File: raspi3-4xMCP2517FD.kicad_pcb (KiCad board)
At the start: 2 copper layers, 25.4 x 53.3 mm, 44 parts, among them J1 Raspberry_Pi_2_3, J2 Conn_02x04_Odd_Even, U1 MCP2517FD-xSL, U2 MCP2517FD-xSL, U3 MCP2517FD-xSL, U4 MCP2517FD-xSL, U5 TJA1049T-3, U6 TJA1049T-3, U7 TJA1049T-3, U8 TJA1049T-3, X1 ASV-20MHz

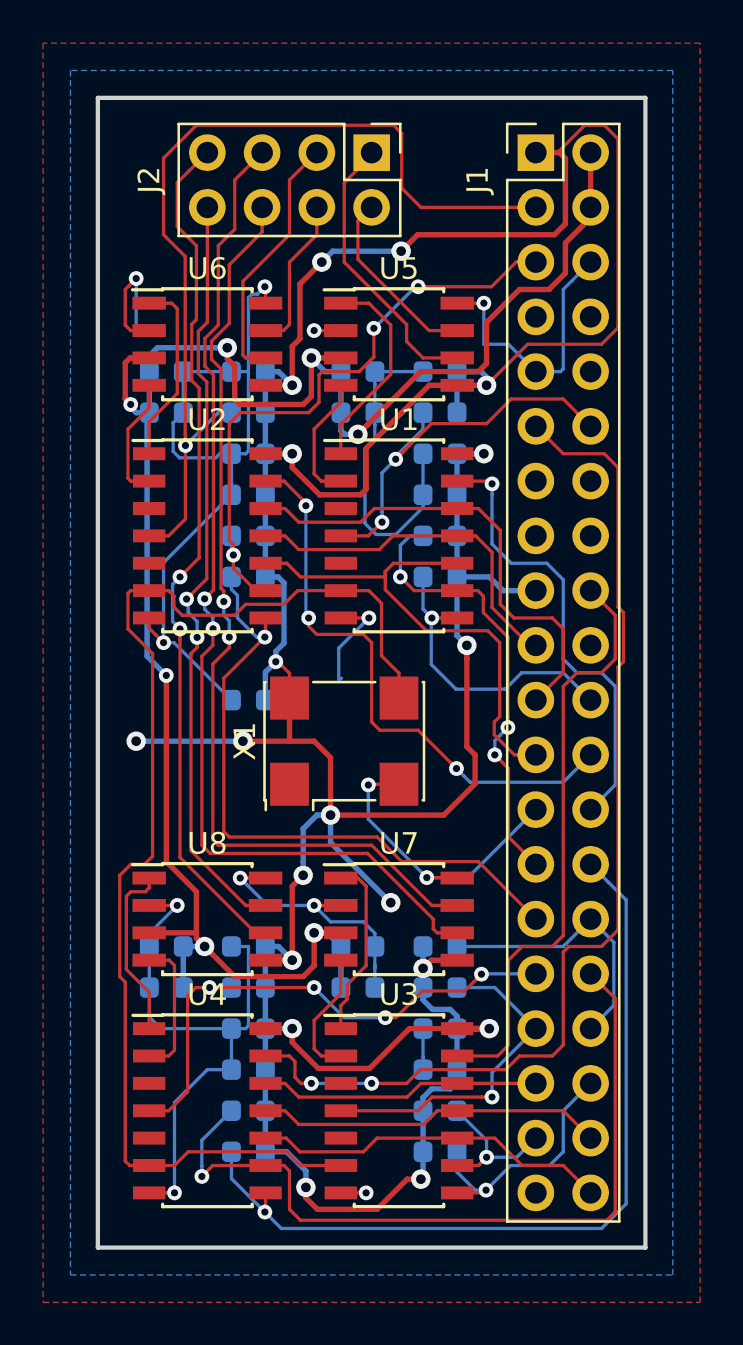
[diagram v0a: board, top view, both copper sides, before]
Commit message: make v2
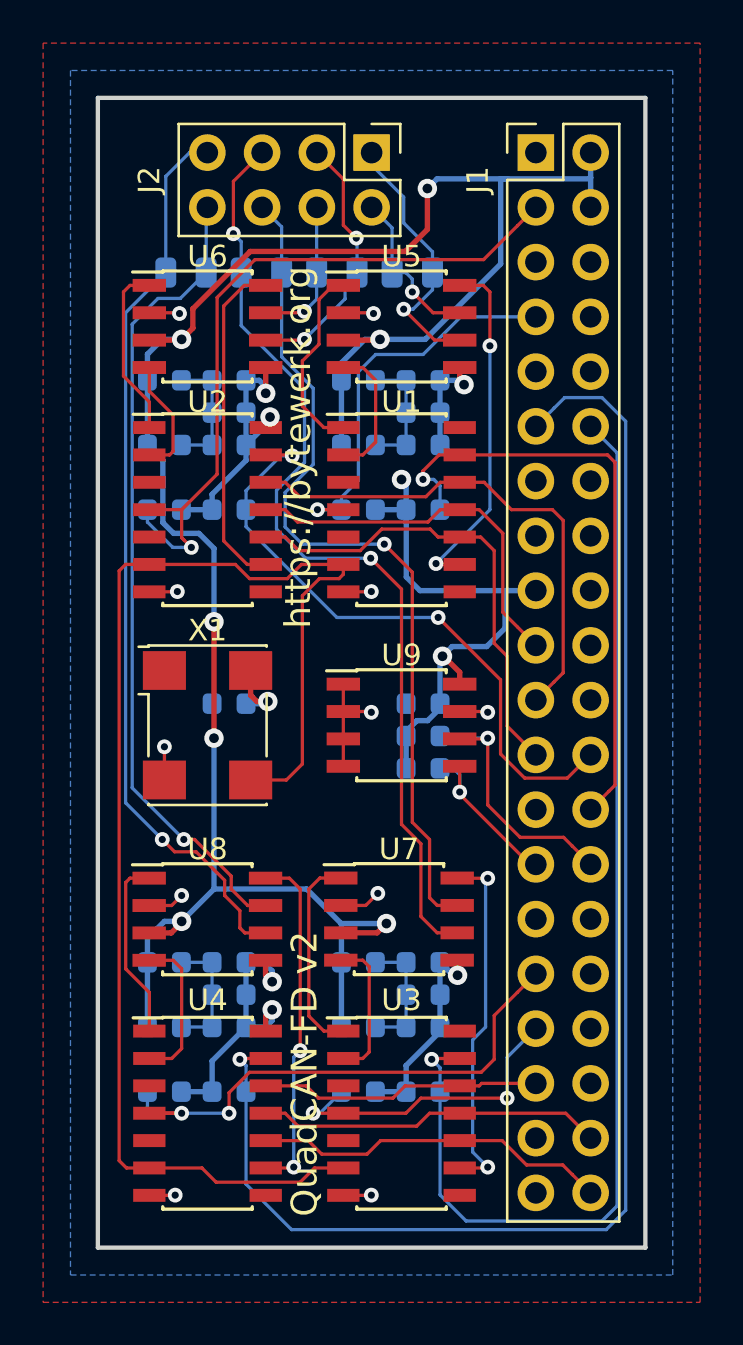
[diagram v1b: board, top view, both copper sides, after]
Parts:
- added C22: 100nF, Capacitor_SMD:C_0603_1608Metric, B.Cu at (87.4, 51.0)
- added R13: dnp, Capacitor_SMD:C_0805_2012Metric, B.Cu at (88.9, 31.0)
- added R14: dnp, Capacitor_SMD:C_0805_2012Metric, B.Cu at (85.4, 31.0)
- added U9: AT24CS32-SSHM, Package_SO:SOIC-8_3.9x4.9mm_P1.27mm, F.Cu at (95.4, 52.0)
- C1, C6, C7, C8: value 100nF -> 1uF
- C18, C19, C20, C21: value 1uF -> 100nF
- R1, R2: value 10K -> 3K9
- R11, R12: value 10K -> dnp; footprint Resistor_SMD:R_0603_1608Metric -> Capacitor_SMD:C_0805_2012Metric
- moved R11 40.8 mm to (95.9, 31.0)
- moved C4 31.7 mm to (84.4, 39.0), turned to 0 degrees
- moved C15 31.3 mm to (96.4, 64.5), turned to 180 degrees
- moved C9 29.7 mm to (96.4, 37.5)
- moved R5 27.9 mm to (87.4, 42.0), turned to 0 degrees
- moved C18 27.7 mm to (87.4, 64.5), turned to 180 degrees
- moved C6 26.9 mm to (93.4, 66.0), turned to 0 degrees
- moved C12 26.6 mm to (87.4, 37.5), turned to 180 degrees
- moved C7 26.6 mm to (87.4, 66.0)
- moved C13 26.3 mm to (87.4, 36.0)
- moved R8 26.1 mm to (93.4, 69.0)
- moved C19 25.7 mm to (87.4, 63.0), turned to 180 degrees
- moved R10 24.2 mm to (84.4, 69.0)
- moved R3 22.2 mm to (96.4, 42.0)
- moved R2 18.4 mm to (96.4, 54.0), turned to 0 degrees
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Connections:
- C11 pad 1: +3V3 -> +5V
- C15 pad 1: +5V -> +3V3
- C16 pad 1: +5V -> +3V3
- C18 pad 1: +5V -> +3V3
- C19 pad 1: +5V -> +3V3
- C2 pad 1: +3V3 -> +5V
- C21 pad 1: +5V -> +3V3
- C4 pad 1: +3V3 -> +5V
- C6 pad 1: +3V3 -> +5V
- C8 pad 1: +3V3 -> +5V
- J1 pad 10: (no net) -> Net-(J1-Pad10)
- J1 pad 12: MCP0_INT -> SPI1_CS0
- J1 pad 13: (no net) -> Net-(J1-Pad13)
- J1 pad 15: (no net) -> Net-(J1-Pad15)
- J1 pad 16: (no net) -> Net-(J1-Pad16)
- J1 pad 18: SPI1_CS0 -> Net-(J1-Pad18)
- J1 pad 22: MCP0_INT1 -> Net-(J1-Pad22)
- J1 pad 27: MCP0_INT0 -> ID_SD
- J1 pad 28: MCP3_INT1 -> ID_SC
- J1 pad 29: MCP1_INT1 -> Net-(J1-Pad29)
- J1 pad 32: MCP3_INT0 -> Net-(J1-Pad32)
- J1 pad 36: MCP2_INT1 -> Net-(J1-Pad36)
- J1 pad 37: MCP2_INT0 -> Net-(J1-Pad37)
- J1 pad 5: MCP1_INT0 -> Net-(J1-Pad5)
- J1 pad 7: (no net) -> MCP0_INT
- J1 pad 8: (no net) -> Net-(J1-Pad8)
- R1 pad 2: MCP3_INT -> ID_SC
- R10 pad 2: MCP1_INT1 -> MCP3_INT
- R11 pad 1: +3V3 -> CAN0_H
- R11 pad 2: MCP2_INT1 -> CAN0_L
- R12 pad 1: +3V3 -> CAN1_H
- R12 pad 2: MCP0_INT1 -> CAN1_L
- R2 pad 2: MCP1_INT -> ID_SD
- R3 pad 2: MCP2_INT -> SPI0_CS0
- R5 pad 2: MCP3_INT0 -> SPI0_CS1
- R6 pad 2: MCP1_INT0 -> MCP1_INT
- R7 pad 2: MCP2_INT0 -> SPI1_CS0
- R8 pad 2: MCP0_INT0 -> MCP2_INT
- R9 pad 2: MCP3_INT1 -> SPI1_CS1
- U1 pad 3: (no net) -> Net-(U1-Pad3)
- U1 pad 5: (no net) -> Net-(U1-Pad5)
- U1 pad 8: MCP0_INT1 -> Net-(U1-Pad8)
- U1 pad 9: MCP0_INT0 -> Net-(U1-Pad9)
- U2 pad 3: (no net) -> Net-(U2-Pad3)
- U2 pad 5: (no net) -> Net-(U2-Pad5)
- U2 pad 8: MCP1_INT1 -> Net-(U2-Pad8)
- U2 pad 9: MCP1_INT0 -> Net-(U2-Pad9)
- U3 pad 3: (no net) -> Net-(U3-Pad3)
- U3 pad 5: (no net) -> Net-(U3-Pad5)
- U3 pad 8: MCP2_INT1 -> Net-(U3-Pad8)
- U3 pad 9: MCP2_INT0 -> Net-(U3-Pad9)
- U4 pad 3: (no net) -> Net-(U4-Pad3)
- U4 pad 5: (no net) -> Net-(U4-Pad5)
- U4 pad 8: MCP3_INT1 -> Net-(U4-Pad8)
- U4 pad 9: MCP3_INT0 -> Net-(U4-Pad9)
- U5 pad 8: GND -> Net-(U1-Pad9)
- U6 pad 8: GND -> Net-(U2-Pad9)
- U7 pad 8: GND -> Net-(U3-Pad9)
- U8 pad 8: GND -> Net-(U4-Pad9)
- X1 pad 1: (no net) -> Net-(X1-Pad1)
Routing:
- net +3V3: track 197.4 -> 70.7 mm, vias 19 -> 9
- net GND: track 145.7 -> 43.0 mm, vias 13 -> 11
- net MCP3_INT1: track 38.3 -> 0.00 mm, vias 1 -> 0
- net MCP3_INT0: track 36.8 -> 0.00 mm, vias 1 -> 0
- net MCP1_INT1: track 31.3 -> 0.00 mm, vias 1 -> 0
- net MCP1_INT0: track 28.5 -> 0.00 mm, vias 3 -> 0
- net SPI1_CS0: track 27.7 -> 53.4 mm, vias 0 -> 1
- net MCP0_INT0: track 20.9 -> 0.00 mm, vias 3 -> 0
- net SPI1_CS1: track 49.1 -> 67.8 mm, vias 2 -> 1
- net Net-(U3-Pad9): track 0.00 -> 16.7 mm, vias 0 -> 2
- net Net-(U1-Pad9): track 0.00 -> 16.3 mm, vias 0 -> 2
- net Net-(U4-Pad9): track 0.00 -> 16.2 mm, vias 0 -> 2
- net Net-(U2-Pad9): track 0.00 -> 15.6 mm
- net MCP0_INT1: track 14.1 -> 0.00 mm, vias 1 -> 0
- net ID_SC: track 0.00 -> 12.6 mm, vias 0 -> 1
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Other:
- board text added: "QuadCAN-FD v2"
- board text added: "https://bytewerk.org"
- board text removed: "4xMCP2517FD RasPi Hat v1.0"
- board text removed: "https://bytewerk.org/"
